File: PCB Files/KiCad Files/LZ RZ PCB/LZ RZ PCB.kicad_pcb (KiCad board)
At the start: 2 copper layers, 63.1 x 8 mm, 5 parts

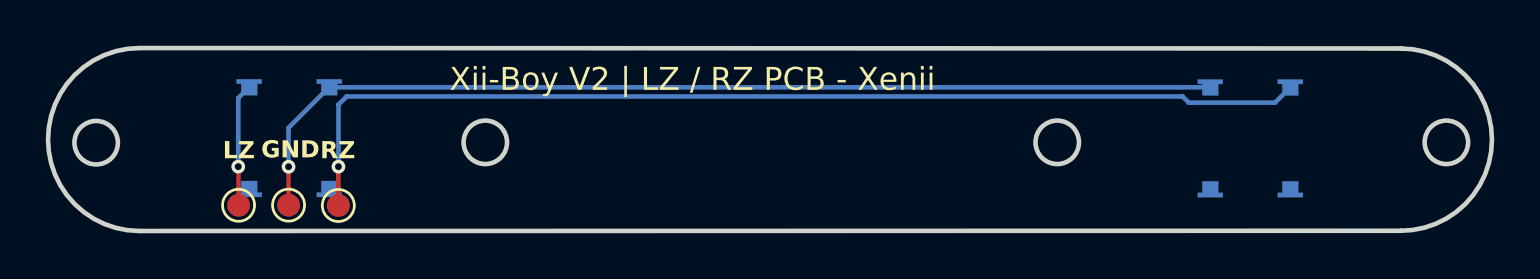
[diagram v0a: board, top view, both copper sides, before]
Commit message: Add files via upload
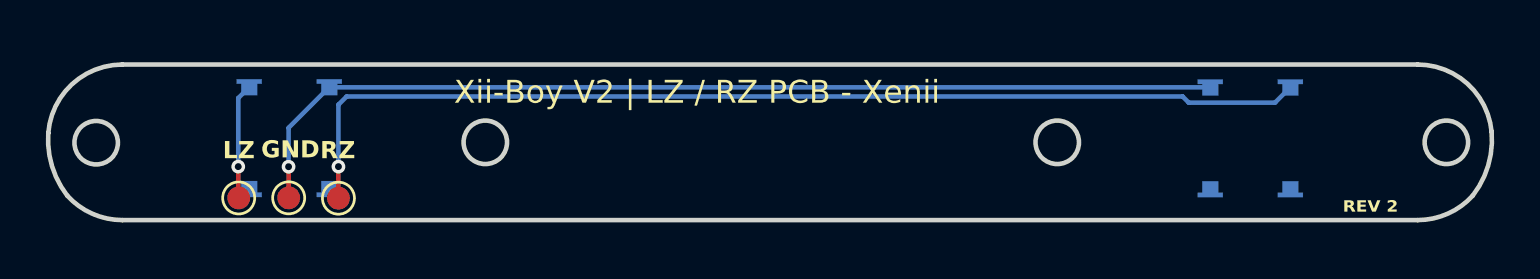
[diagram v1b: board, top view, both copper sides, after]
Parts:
- moved TP1 0.32 mm to (46.1, 58.3)
- moved TP3 0.32 mm to (50.5, 58.3)
- moved TP2 0.32 mm to (48.3, 58.3)
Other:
- board size 63.1 x 8 mm -> 63.1 x 6.8 mm
- board text added: "REV 2"
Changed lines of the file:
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@@
 			(drillshape 0)
 			(scaleselection 1)
-			(outputdirectory "../../../Xii-Boy V2/Gerber/Z-PCB/")
+			(outputdirectory "../../Gerber/Z-PCB/")
 		)
 	)
@@
 	(footprint "TestPoint:TestPoint_Pad_D1.0mm"
 		(layer "F.Cu")
-		(at 50.445 58.595)
+		(at 50.45 58.275)
 		(descr "SMD pad as test Point, diameter 1.0mm")
 		(tags "test point SMD pad")
@@
 	(footprint "TestPoint:TestPoint_Pad_D1.0mm"
 		(layer "F.Cu")
-		(at 48.27 58.58)
+		(at 48.275 58.26)
 		(descr "SMD pad as test Point, diameter 1.0mm")
 		(tags "test point SMD pad")
@@
 	(footprint "TestPoint:TestPoint_Pad_D1.0mm"
 		(layer "F.Cu")
-		(at 46.085 58.585)
+		(at 46.09 58.265)
 		(descr "SMD pad as test Point, diameter 1.0mm")
 		(tags "test point SMD pad")
@@
 	)
 	(gr_line
-		(start 41.755724 59.700001)
-		(end 96.889432 59.69)
-		(stroke
-			(width 0.2)
-			(type default)
-		)
-		(layer "Dwgs.User")
-	)
-	(gr_line
-		(start 96.890154 51.722589)
-		(end 41.750126 51.702588)
-		(stroke
-			(width 0.2)
-			(type default)
-		)
-		(layer "Dwgs.User")
-	)
-	(gr_arc
-		(start 96.890154 51.722589)
-		(mid 100.872414 55.706655)
-		(end 96.889432 59.69)
-		(stroke
-			(width 0.2)
-			(type default)
-		)
-		(layer "Dwgs.User")
-	)
-	(gr_circle
-		(center 90.289466 55.672243)
-		(end 90.289466 54.172243)
-		(stroke
-			(width 0.2)
-			(type default)
-		)
-		(fill none)
-		(layer "Dwgs.User")
-	)
-	(gr_arc
-		(start 41.755724 59.700001)
-		(mid 37.756293 55.704093)
-		(end 41.750126 51.702588)
-		(stroke
-			(width 0.2)
-			(type default)
-		)
-		(layer "Dwgs.User")
-	)
-	(gr_circle
-		(center 39.86 55.84)
-		(end 39.86 54.89)
-		(stroke
-			(width 0.2)
-			(type default)
-		)
-		(fill none)
-		(layer "Dwgs.User")
-	)
-	(gr_circle
-		(center 81.87 55.823303)
-		(end 81.87 54.873303)
-		(stroke
-			(width 0.2)
-			(type default)
-		)
-		(fill none)
-		(layer "Dwgs.User")
-	)
-	(gr_line
 		(start 50.455 58.575)
 		(end 46.085 58.585)
@@
 		(layer "Dwgs.User")
 	)
-	(gr_circle
-		(center 48.289466 55.672243)
-		(end 48.289466 54.172243)
+	(gr_arc
+		(start 41.0063 59.233303)
+		(mid 39.689764 58.954706)
+		(end 38.598938 58.166682)
 		(stroke
 			(width 0.2)
 			(type default)
 		)
-		(fill none)
-		(layer "Dwgs.User")
-	)
-	(gr_circle
-		(center 98.88 55.823303)
-		(end 98.88 54.873303)
-		(stroke
-			(width 0.2)
-			(type default)
-		)
-		(fill none)
-		(layer "Dwgs.User")
-	)
-	(gr_circle
-		(center 56.87 55.823303)
-		(end 56.87 54.873303)
-		(stroke
-			(width 0.2)
-			(type default)
-		)
-		(fill none)
-		(layer "Dwgs.User")
-	)
-	(gr_line
-		(start 96.890154 51.732589)
-		(end 41.750126 51.712588)
+		(layer "Edge.Cuts")
+	)
+	(gr_arc
+		(start 100.857855 55.376027)
+		(mid 100.707606 56.850281)
+		(end 100.028917 58.16762)
 		(stroke
 			(width 0.2)
@@
 		(layer "Edge.Cuts")
 	)
+	(gr_circle
+		(center 81.87 55.833303)
+		(end 81.87 54.883303)
+		(stroke
+			(width 0.2)
+			(type default)
+		)
+		(fill none)
+		(layer "Edge.Cuts")
+	)
 	(gr_arc
-		(start 41.755724 59.710001)
-		(mid 37.756293 55.714093)
-		(end 41.750126 51.712588)
+		(start 100.028917 58.16762)
+		(mid 98.941216 58.953703)
+		(end 97.628645 59.233303)
+		(stroke
+			(width 0.2)
+			(type default)
+		)
+		(layer "Edge.Cuts")
+	)
+	(gr_arc
+		(start 37.766381 55.427412)
+		(mid 38.796663 53.300007)
+		(end 40.995789 52.433303)
+		(stroke
+			(width 0.2)
+			(type default)
+		)
+		(layer "Edge.Cuts")
+	)
+	(gr_arc
+		(start 97.6224 52.433303)
+		(mid 99.809159 53.279022)
+		(end 100.857855 55.376027)
+		(stroke
+			(width 0.2)
+			(type default)
+		)
+		(layer "Edge.Cuts")
+	)
+	(gr_arc
+		(start 38.598938 58.166682)
+		(mid 37.9291 56.874112)
+		(end 37.766381 55.427412)
+		(stroke
+			(width 0.2)
+			(type default)
+		)
+		(layer "Edge.Cuts")
+	)
+	(gr_line
+		(start 97.6224 52.433303)
+		(end 40.995789 52.433303)
 		(stroke
 			(width 0.2)
@@
 		(layer "Edge.Cuts")
 	)
-	(gr_line
-		(start 41.755724 59.710001)
-		(end 96.889432 59.7)
-		(stroke
-			(width 0.2)
-			(type default)
-		)
-		(layer "Edge.Cuts")
-	)
-	(gr_arc
-		(start 96.890154 51.732589)
-		(mid 100.872414 55.716655)
-		(end 96.889432 59.7)
-		(stroke
-			(width 0.2)
-			(type default)
-		)
-		(layer "Edge.Cuts")
-	)
-	(gr_circle
-		(center 81.87 55.833303)
-		(end 81.87 54.883303)
-		(stroke
-			(width 0.2)
-			(type default)
-		)
-		(fill none)
-		(layer "Edge.Cuts")
-	)
 	(gr_circle
 		(center 39.86 55.85)
@@
 		)
 		(fill none)
+		(layer "Edge.Cuts")
+	)
+	(gr_line
+		(start 41.0063 59.233303)
+		(end 97.628645 59.233303)
+		(stroke
+			(width 0.2)
+			(type default)
+		)
 		(layer "Edge.Cuts")
 	)
@@
 		)
 	)
+	(gr_text "REV 2"
+		(at 94.35 58.925 0)
+		(layer "F.SilkS")
+		(effects
+			(font
+				(size 0.5 0.54)
+				(thickness 0.125)
+				(bold yes)
+			)
+			(justify left bottom)
+		)
+	)
 	(gr_text "GND"
 		(at 47.07 56.585 0)
@@
 	)
 	(gr_text "Xii-Boy V2 | LZ / RZ PCB - Xenii"
-		(at 55.3 53.66 0)
+		(at 55.5 54.225 0)
 		(layer "F.SilkS")
 		(effects
@@
 	)
 	(segment
-		(start 46.085 56.911)
-		(end 46.085 58.585)
+		(start 46.07 56.896)
+		(end 46.085 56.911)
 		(width 0.2)
 		(layer "F.Cu")
@@
 	)
 	(segment
+		(start 46.07 58.245)
+		(end 46.09 58.265)
+		(width 0.2)
+		(layer "F.Cu")
+		(net 1)
+	)
+	(segment
 		(start 46.07 56.896)
-		(end 46.085 56.911)
+		(end 46.07 58.245)
 		(width 0.2)
 		(layer "F.Cu")
@@
 	)
 	(segment
+		(start 48.27 56.899998)
+		(end 48.27 58.255)
+		(width 0.2)
+		(layer "F.Cu")
+		(net 2)
+	)
+	(segment
 		(start 48.27 58.58)
+		(end 48.275 58.575)
+		(width 0.2)
+		(layer "F.Cu")
+		(net 2)
+	)
+	(segment
+		(start 48.275 56.904998)
 		(end 48.27 56.899998)
+		(width 0.2)
+		(layer "F.Cu")
+		(net 2)
+	)
+	(segment
+		(start 48.27 58.255)
+		(end 48.275 58.26)
 		(width 0.2)
 		(layer "F.Cu")
@@
 	)
 	(segment
-		(start 50.445 56.901)
-		(end 50.445 58.595)
+		(start 50.45 56.896)
+		(end 50.45 58.275)
 		(width 0.2)
 		(layer "F.Cu")
@@
 	)
 	(group ""
-		(members "1dc31bb0-c5f6-4b2d-a6b3-dffee8842ee5" "256e2616-c87f-4e44-a893-d500a289a8e6"
-			"35af1e81-50d6-41e1-9c34-fac73d4beb4e" "4094e23e-99e7-4cb9-9684-339d3a7ff784"
-			"4da462d9-40b5-4da9-a1aa-23bf201a3119" "4f83917b-6136-49b0-953a-e546e3664265"
-			"5fc76100-2e70-4b2a-8d7f-ef27e9c8df35" "ba9098ce-5895-40e5-80b0-2cc3e22440e5"
-			"d37795d1-7ae0-43cf-8128-27e97aa07487" "eddd539c-c717-483b-8a90-ea6e367d6848"
-		)
-	)
-	(group ""
-		(members "2558a037-f90f-4277-b805-083862776a0c" "2d8d4c40-98c0-4423-a483-4919030f6107"
-			"3c7a4163-9be0-46b3-9dab-3b7ab511b238" "4d6bcea3-839a-45a7-ba8d-7cbf0e1de618"
-			"71c3d7bc-39f9-4e30-afbc-48e61bfc55e6" "86b14903-f4c7-4ebc-b6a8-870c56a2b2f7"
-			"888504f5-fd56-40ed-95bb-a62add055d78" "9395b4b1-49ef-4d56-bcc6-84070c390f27"
-		)
-	)
+		(members "37d1e020-8ebf-4d77-a35a-9041e4899b6f" "71bc99a3-4280-4085-9e18-ea6ebe885f90"
+			"8210ac55-5732-44dd-b752-bf411bda267b" "929fc8e7-a216-487d-8b53-167ef837f2e0"
+			"95223d07-f29b-444e-a74d-e5fc31fe6fd5" "9faf1cdb-1c34-41e0-aa03-4d65d2352ed0"
+			"af1566e6-49b3-45ec-9596-4a25f70b6945" "b1ee829c-0ca3-42d7-8dc9-052be9a270c0"
+			"c6eda574-4154-4a47-8e58-8ec95779e60a" "da4892fa-7181-4c1e-9a02-1b22f28559f5"
+			"dca183da-2769-4ac9-8bd5-7dac7e310fc7" "fa11f398-894e-4831-b050-7af8e765d387"
+		)
+	)
